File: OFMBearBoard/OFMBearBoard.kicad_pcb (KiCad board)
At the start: 2 copper layers, 50 x 65.5 mm, 15 parts, among them J1 X Motor, J2 Y Motor, J3 Z Motor, J4 LED, J5 5V, U1 ULN2003APG, U2 ULN2003APG

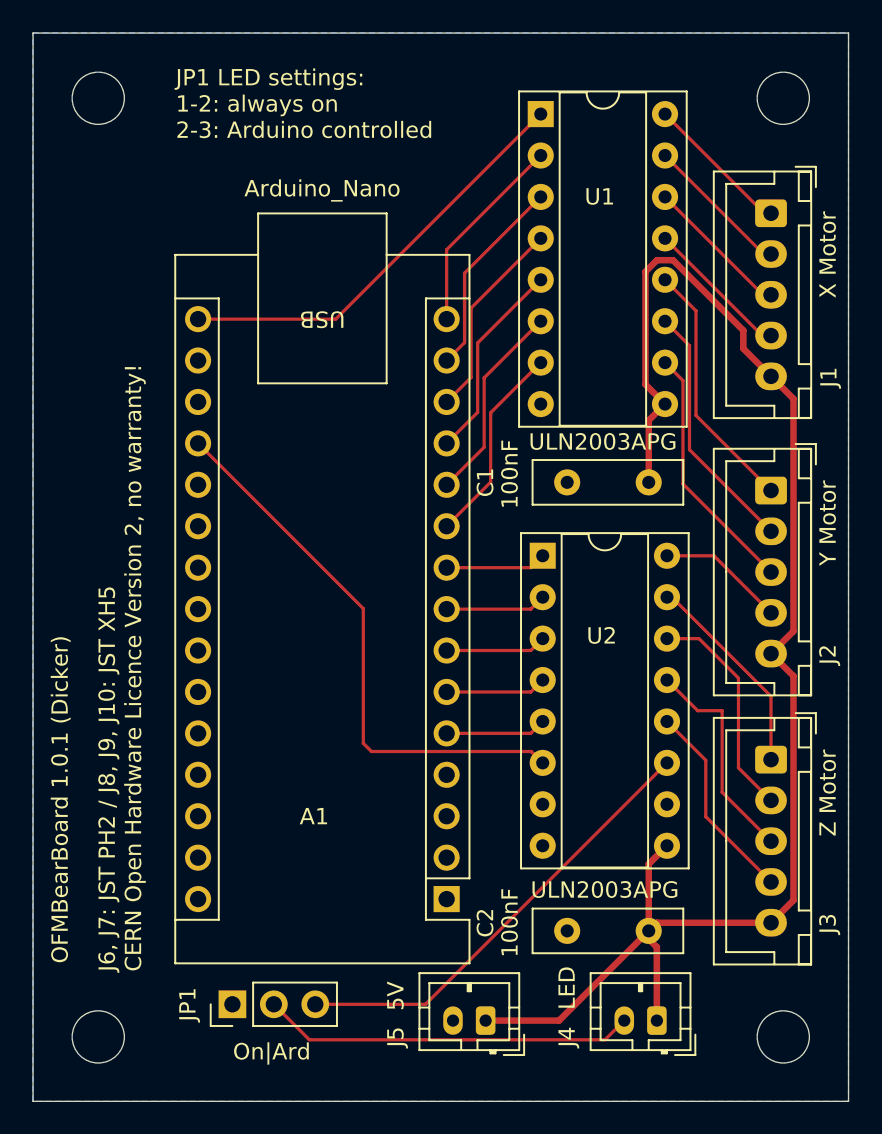
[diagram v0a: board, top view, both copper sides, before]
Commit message: New Gerber Zip
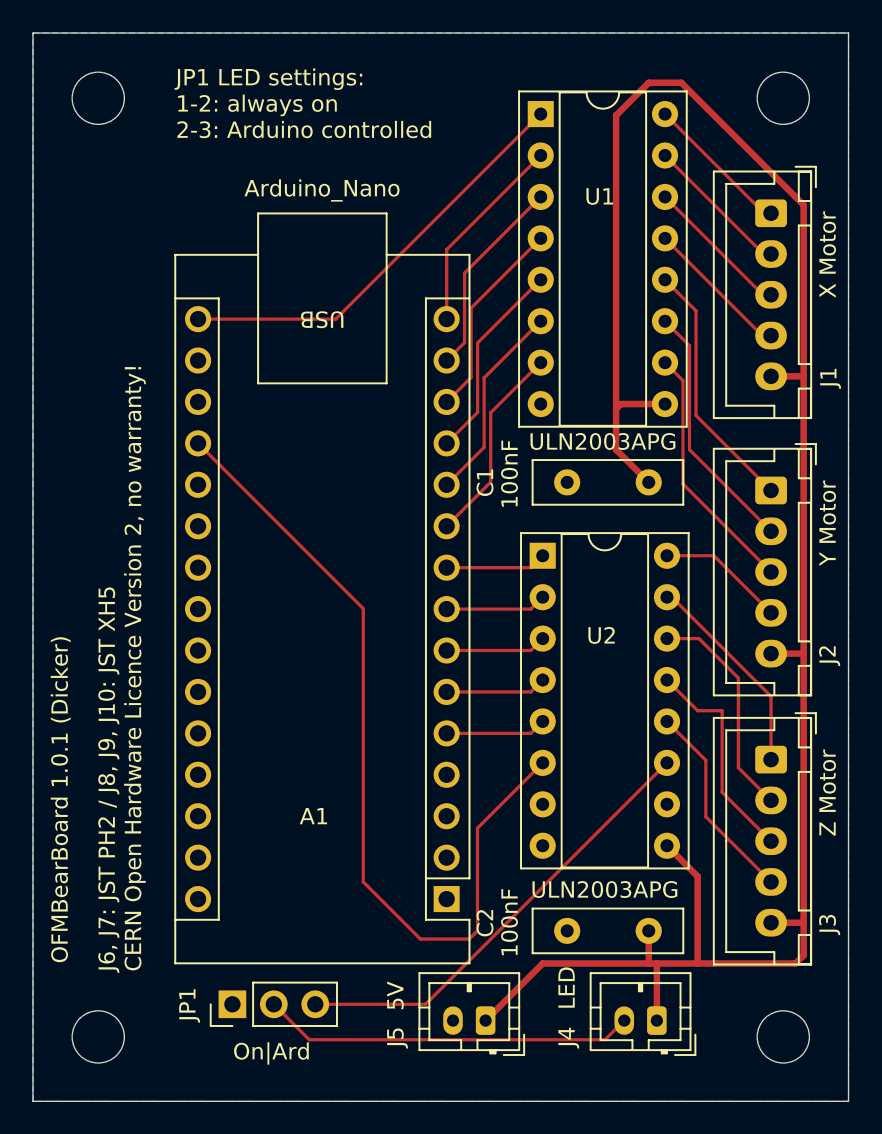
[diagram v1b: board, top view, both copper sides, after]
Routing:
- net +5V: track 92.6 -> 128.5 mm
- net /A00: track 34.1 -> 51.7 mm
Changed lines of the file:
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@@
-	)
-	(segment
-		(start 109.8 65.5)
-		(end 100 65.5)
-		(width 0.2)
-		(layer "F.Cu")
-		(net 16)
-	)
-	(segment
-		(start 100 65.5)
-		(end 99.5 65)
-		(width 0.2)
-		(layer "F.Cu")
-		(net 16)
 	)
 	(segment
 		(start 99.5 56.74)
-		(end 89.37 46.61)
-		(width 0.2)
-		(layer "F.Cu")
-		(net 16)
-	)
-	(segment
-		(start 99.5 65)
+		(end 99.5 73.5)
+		(width 0.2)
+		(layer "F.Cu")
+		(net 16)
+	)
+	(segment
+		(start 99.5 73.5)
+		(end 103 77)
+		(width 0.2)
+		(layer "F.Cu")
+		(net 16)
+	)
+	(segment
+		(start 89.37 46.61)
 		(end 99.5 56.74)
 		(width 0.2)
@@
 	)
 	(segment
-		(start 110.5 66.2)
-		(end 109.8 65.5)
-		(width 0.2)
-		(layer "F.Cu")
-		(net 16)
-	)
-	(segment
-		(start 117.502943 35.38)
-		(end 118.497057 35.38)
-		(width 0.4)
-		(layer "F.Cu")
-		(net 18)
-	)
-	(segment
-		(start 122.8 39.682943)
-		(end 122.8 40.8)
-		(width 0.4)
-		(layer "F.Cu")
-		(net 18)
-	)
-	(segment
-		(start 122.8 40.8)
+		(start 103 77)
+		(end 106 77)
+		(width 0.2)
+		(layer "F.Cu")
+		(net 16)
+	)
+	(segment
+		(start 106.5 70.2)
+		(end 110.5 66.2)
+		(width 0.2)
+		(layer "F.Cu")
+		(net 16)
+	)
+	(segment
+		(start 106.5 76.5)
+		(end 106.5 70.2)
+		(width 0.2)
+		(layer "F.Cu")
+		(net 16)
+	)
+	(segment
+		(start 106 77)
+		(end 106.5 76.5)
+		(width 0.2)
+		(layer "F.Cu")
+		(net 16)
+	)
+	(segment
+		(start 118 44.2)
+		(end 115.3 44.2)
+		(width 0.4)
+		(layer "F.Cu")
+		(net 18)
+	)
+	(segment
+		(start 115 26.5)
+		(end 117 24.5)
+		(width 0.4)
+		(layer "F.Cu")
+		(net 18)
+	)
+	(segment
+		(start 117.5 78.5)
+		(end 117 78.5)
+		(width 0.4)
+		(layer "F.Cu")
+		(net 18)
+	)
+	(segment
+		(start 115.3 44.2)
+		(end 115 44.5)
+		(width 0.4)
+		(layer "F.Cu")
+		(net 18)
+	)
+	(segment
+		(start 126 78.5)
+		(end 120 78.5)
+		(width 0.4)
+		(layer "F.Cu")
+		(net 18)
+	)
+	(segment
+		(start 115 44.5)
+		(end 115 26.5)
+		(width 0.4)
+		(layer "F.Cu")
+		(net 18)
+	)
+	(segment
+		(start 117 24.5)
+		(end 119 24.5)
+		(width 0.4)
+		(layer "F.Cu")
+		(net 18)
+	)
+	(segment
+		(start 124.5 59.5)
+		(end 126.5 59.5)
+		(width 0.4)
+		(layer "F.Cu")
+		(net 18)
+	)
+	(segment
+		(start 124.5 76)
+		(end 126.5 76)
+		(width 0.4)
+		(layer "F.Cu")
+		(net 18)
+	)
+	(segment
+		(start 126.5 76)
+		(end 126.5 78)
+		(width 0.4)
+		(layer "F.Cu")
+		(net 18)
+	)
+	(segment
+		(start 120 73.16)
+		(end 120 78.5)
+		(width 0.4)
+		(layer "F.Cu")
+		(net 18)
+	)
+	(segment
+		(start 110.5 78.5)
+		(end 107 82)
+		(width 0.4)
+		(layer "F.Cu")
+		(net 18)
+	)
+	(segment
+		(start 117.5 82)
+		(end 117.5 78.5)
+		(width 0.4)
+		(layer "F.Cu")
+		(net 18)
+	)
+	(segment
+		(start 115 47)
+		(end 117 49)
+		(width 0.4)
+		(layer "F.Cu")
+		(net 18)
+	)
+	(segment
+		(start 126.5 42.5)
+		(end 126.5 32)
+		(width 0.4)
+		(layer "F.Cu")
+		(net 18)
+	)
+	(segment
+		(start 126.5 78)
+		(end 126 78.5)
+		(width 0.4)
+		(layer "F.Cu")
+		(net 18)
+	)
+	(segment
+		(start 118.12 71.28)
+		(end 120 73.16)
+		(width 0.4)
+		(layer "F.Cu")
+		(net 18)
+	)
+	(segment
+		(start 120 78.5)
+		(end 117.5 78.5)
+		(width 0.4)
+		(layer "F.Cu")
+		(net 18)
+	)
+	(segment
+		(start 117 76.5)
+		(end 117 78.5)
+		(width 0.4)
+		(layer "F.Cu")
+		(net 18)
+	)
+	(segment
+		(start 126.5 59.5)
+		(end 126.5 76)
+		(width 0.4)
+		(layer "F.Cu")
+		(net 18)
+	)
+	(segment
+		(start 117 78.5)
+		(end 110.5 78.5)
+		(width 0.4)
+		(layer "F.Cu")
+		(net 18)
+	)
+	(segment
+		(start 126.5 42.5)
+		(end 126.5 59.5)
+		(width 0.4)
+		(layer "F.Cu")
+		(net 18)
+	)
+	(segment
+		(start 115 44.5)
+		(end 115 47)
+		(width 0.4)
+		(layer "F.Cu")
+		(net 18)
+	)
+	(segment
+		(start 119 24.5)
+		(end 126.5 32)
+		(width 0.4)
+		(layer "F.Cu")
+		(net 18)
+	)
+	(segment
+		(start 126.5 42.5)
 		(end 124.5 42.5)
 		(width 0.4)
 		(layer "F.Cu")
-		(net 18)
-	)
-	(segment
-		(start 117 45.2)
-		(end 118 44.2)
-		(width 0.4)
-		(layer "F.Cu")
-		(net 18)
-	)
-	(segment
-		(start 117 49)
-		(end 117 45.2)
-		(width 0.4)
-		(layer "F.Cu")
-		(net 18)
-	)
-	(segment
-		(start 118 44.2)
-		(end 116.8 43)
-		(width 0.4)
-		(layer "F.Cu")
-		(net 18)
-	)
-	(segment
-		(start 117 77)
-		(end 117.5 77.5)
-		(width 0.4)
-		(layer "F.Cu")
-		(net 18)
-	)
-	(segment
-		(start 125.875 43.875)
-		(end 124.5 42.5)
-		(width 0.4)
-		(layer "F.Cu")
-		(net 18)
-	)
-	(segment
-		(start 107 82)
-		(end 111.5 82)
-		(width 0.4)
-		(layer "F.Cu")
-		(net 18)
-	)
-	(segment
-		(start 117 76.5)
-		(end 117 72.4)
-		(width 0.4)
-		(layer "F.Cu")
-		(net 18)
-	)
-	(segment
-		(start 117 76.5)
-		(end 117 77)
-		(width 0.4)
-		(layer "F.Cu")
-		(net 18)
-	)
-	(segment
-		(start 124.5 76)
-		(end 117.5 76)
-		(width 0.4)
-		(layer "F.Cu")
-		(net 18)
-	)
-	(segment
-		(start 125.875 60.875)
-		(end 124.5 59.5)
-		(width 0.4)
-		(layer "F.Cu")
-		(net 18)
-	)
-	(segment
-		(start 125.875 58.125)
-		(end 125.875 43.875)
-		(width 0.4)
-		(layer "F.Cu")
-		(net 18)
-	)
-	(segment
-		(start 117.5 76)
-		(end 117 76.5)
-		(width 0.4)
-		(layer "F.Cu")
-		(net 18)
-	)
-	(segment
-		(start 124.5 76)
-		(end 125.875 74.625)
-		(width 0.4)
-		(layer "F.Cu")
-		(net 18)
-	)
-	(segment
-		(start 116.8 36.082943)
-		(end 117.502943 35.38)
-		(width 0.4)
-		(layer "F.Cu")
-		(net 18)
-	)
-	(segment
-		(start 117 72.4)
-		(end 118.12 71.28)
-		(width 0.4)
-		(layer "F.Cu")
-		(net 18)
-	)
-	(segment
-		(start 118.497057 35.38)
-		(end 122.8 39.682943)
-		(width 0.4)
-		(layer "F.Cu")
-		(net 18)
-	)
-	(segment
-		(start 124.5 59.5)
-		(end 125.875 58.125)
-		(width 0.4)
-		(layer "F.Cu")
-		(net 18)
-	)
-	(segment
-		(start 117.5 77.5)
-		(end 117.5 82)
-		(width 0.4)
-		(layer "F.Cu")
-		(net 18)
-	)
-	(segment
-		(start 125.875 74.625)
-		(end 125.875 60.875)
-		(width 0.4)
-		(layer "F.Cu")
-		(net 18)
-	)
-	(segment
-		(start 116.8 43)
-		(end 116.8 36.082943)
-		(width 0.4)
-		(layer "F.Cu")
-		(net 18)
-	)
-	(segment
-		(start 111.5 82)
-		(end 117 76.5)
-		(width 0.4)
-		(layer "F.Cu")
